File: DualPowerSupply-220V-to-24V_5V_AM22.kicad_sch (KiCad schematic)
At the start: 7 parts, among them U1 AM22-24W2405V

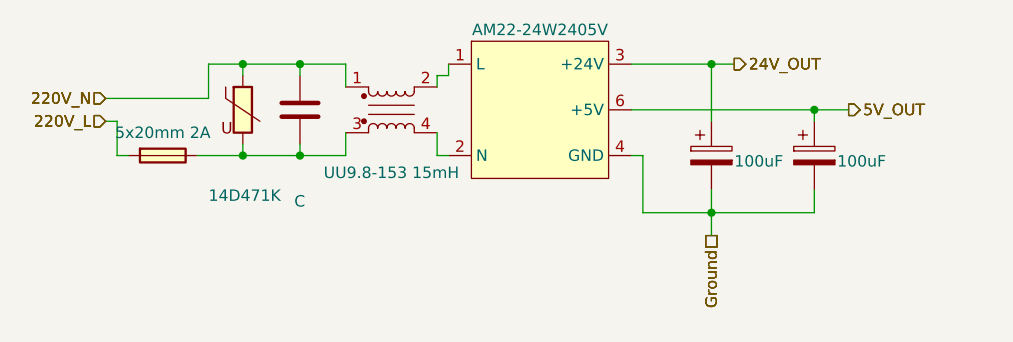
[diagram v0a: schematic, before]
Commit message: layout p1
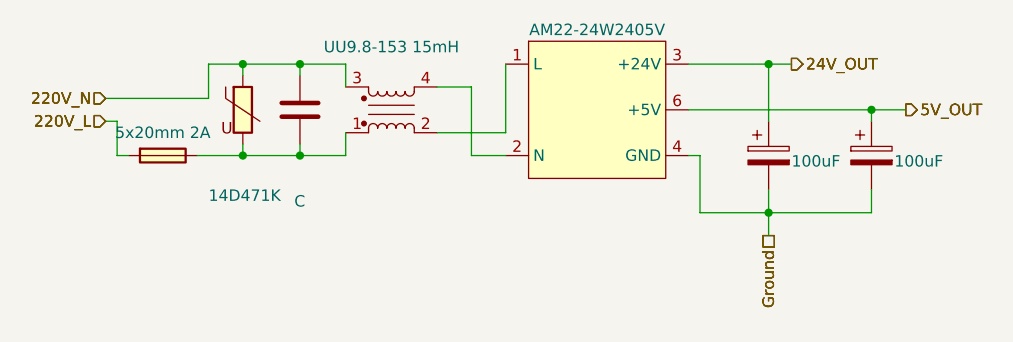
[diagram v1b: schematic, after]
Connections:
- net 220V_N: now also FL1.3; no longer FL1.1
- net at C1.2, F1.2, RV1.2: now also FL1.1; no longer FL1.3
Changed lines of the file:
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@@
 	)
 	(junction
-		(at 157.48 107.95)
+		(at 163.83 107.95)
 		(diameter 0)
 		(color 0 0 0 0)
@@
 	)
 	(junction
-		(at 157.48 91.44)
+		(at 163.83 91.44)
 		(diameter 0)
 		(color 0 0 0 0)
 	)
 	(junction
-		(at 168.91 96.52)
+		(at 175.26 96.52)
 		(diameter 0)
 		(color 0 0 0 0)
@@
 	(wire
 		(pts
-			(xy 127 92.71) (xy 127 93.98)
-		)
-		(stroke
-			(width 0)
-			(type default)
-		)
-	)
-	(wire
-		(pts
-			(xy 148.59 96.52) (xy 168.91 96.52)
+			(xy 154.94 96.52) (xy 175.26 96.52)
 		)
 		(stroke
@@
 	(wire
 		(pts
-			(xy 149.86 107.95) (xy 149.86 101.6)
+			(xy 156.21 107.95) (xy 156.21 101.6)
 		)
 		(stroke
@@
 	(wire
 		(pts
-			(xy 127 92.71) (xy 128.27 92.71)
-		)
-		(stroke
-			(width 0)
-			(type default)
-		)
-	)
-	(wire
-		(pts
-			(xy 160.02 91.44) (xy 157.48 91.44)
-		)
-		(stroke
-			(width 0)
-			(type default)
-		)
-	)
-	(wire
-		(pts
-			(xy 127 99.06) (xy 127 101.6)
-		)
-		(stroke
-			(width 0)
-			(type default)
-		)
-	)
-	(wire
-		(pts
-			(xy 127 101.6) (xy 128.27 101.6)
-		)
-		(stroke
-			(width 0)
-			(type default)
-		)
-	)
-	(wire
-		(pts
-			(xy 128.27 92.71) (xy 128.27 91.44)
+			(xy 166.37 91.44) (xy 163.83 91.44)
+		)
+		(stroke
+			(width 0)
+			(type default)
+		)
+	)
+	(wire
+		(pts
+			(xy 130.81 93.98) (xy 130.81 101.6)
+		)
+		(stroke
+			(width 0)
+			(type default)
+		)
+	)
+	(wire
+		(pts
+			(xy 127 99.06) (xy 134.62 99.06)
 		)
 		(stroke
@@
 	(wire
 		(pts
+			(xy 127 93.98) (xy 130.81 93.98)
+		)
+		(stroke
+			(width 0)
+			(type default)
+		)
+	)
+	(wire
+		(pts
 			(xy 111.76 100.33) (xy 111.76 101.6)
 		)
@@
 	(wire
 		(pts
-			(xy 157.48 91.44) (xy 157.48 97.79)
-		)
-		(stroke
-			(width 0)
-			(type default)
-		)
-	)
-	(wire
-		(pts
-			(xy 168.91 96.52) (xy 168.91 97.79)
+			(xy 163.83 91.44) (xy 163.83 97.79)
+		)
+		(stroke
+			(width 0)
+			(type default)
+		)
+	)
+	(wire
+		(pts
+			(xy 175.26 96.52) (xy 175.26 97.79)
 		)
 		(stroke
@@
 	(wire
 		(pts
-			(xy 157.48 105.41) (xy 157.48 107.95)
-		)
-		(stroke
-			(width 0)
-			(type default)
-		)
-	)
-	(wire
-		(pts
-			(xy 168.91 105.41) (xy 168.91 107.95)
-		)
-		(stroke
-			(width 0)
-			(type default)
-		)
-	)
-	(wire
-		(pts
-			(xy 148.59 91.44) (xy 157.48 91.44)
+			(xy 163.83 105.41) (xy 163.83 107.95)
+		)
+		(stroke
+			(width 0)
+			(type default)
+		)
+	)
+	(wire
+		(pts
+			(xy 175.26 105.41) (xy 175.26 107.95)
+		)
+		(stroke
+			(width 0)
+			(type default)
+		)
+	)
+	(wire
+		(pts
+			(xy 154.94 91.44) (xy 163.83 91.44)
 		)
 		(stroke
@@
 	(wire
 		(pts
-			(xy 157.48 107.95) (xy 157.48 110.49)
+			(xy 163.83 107.95) (xy 163.83 110.49)
+		)
+		(stroke
+			(width 0)
+			(type default)
+		)
+	)
+	(wire
+		(pts
+			(xy 134.62 99.06) (xy 134.62 91.44)
 		)
 		(stroke
@@
 	(wire
 		(pts
-			(xy 168.91 96.52) (xy 172.72 96.52)
-		)
-		(stroke
-			(width 0)
-			(type default)
-		)
-	)
-	(wire
-		(pts
-			(xy 149.86 101.6) (xy 148.59 101.6)
-		)
-		(stroke
-			(width 0)
-			(type default)
-		)
-	)
-	(wire
-		(pts
-			(xy 168.91 107.95) (xy 157.48 107.95)
+			(xy 130.81 101.6) (xy 134.62 101.6)
+		)
+		(stroke
+			(width 0)
+			(type default)
+		)
+	)
+	(wire
+		(pts
+			(xy 175.26 96.52) (xy 179.07 96.52)
+		)
+		(stroke
+			(width 0)
+			(type default)
+		)
+	)
+	(wire
+		(pts
+			(xy 156.21 101.6) (xy 154.94 101.6)
+		)
+		(stroke
+			(width 0)
+			(type default)
+		)
+	)
+	(wire
+		(pts
+			(xy 175.26 107.95) (xy 163.83 107.95)
 		)
 		(stroke
@@
 	(wire
 		(pts
-			(xy 149.86 107.95) (xy 157.48 107.95)
+			(xy 156.21 107.95) (xy 163.83 107.95)
 		)
 		(stroke
@@
 	(hierarchical_label "24V_OUT"
 		(shape output)
-		(at 160.02 91.44 0)
+		(at 166.37 91.44 0)
 		(fields_autoplaced yes)
 		(effects
@@
 	(hierarchical_label "24V_OUT"
 		(shape output)
-		(at 160.02 91.44 0)
+		(at 166.37 91.44 0)
 		(fields_autoplaced yes)
 		(effects
@@
 	(hierarchical_label "Ground"
 		(shape passive)
-		(at 157.48 110.49 270)
+		(at 163.83 110.49 270)
 		(fields_autoplaced yes)
 		(effects
@@
 	(hierarchical_label "Ground"
 		(shape passive)
-		(at 157.48 110.49 270)
+		(at 163.83 110.49 270)
 		(fields_autoplaced yes)
 		(effects
@@
 	(hierarchical_label "5V_OUT"
 		(shape output)
-		(at 172.72 96.52 0)
+		(at 179.07 96.52 0)
 		(fields_autoplaced yes)
 		(effects
@@
 	(hierarchical_label "5V_OUT"
 		(shape output)
-		(at 172.72 96.52 0)
+		(at 179.07 96.52 0)
 		(fields_autoplaced yes)
 		(effects
@@
 		(lib_id "IVS_SYMBOLS:Filter_EMI_LL")
 		(at 121.92 96.52 0)
+		(mirror x)
 		(unit 1)
 		(exclude_from_sim no)
@@
 		(dnp no)
 		(property "Reference" "FL1"
-			(at 121.92 100.965 0)
+			(at 121.92 92.075 0)
 			(effects
 				(font
@@
 		)
 		(property "Value" "UU9.8-153 15mH"
-			(at 121.92 103.505 0)
+			(at 121.92 89.535 0)
 			(effects
 				(font
@@
 		)
 		(property "Footprint" "SpiritBoi_Footprint_Library:ACFilterChoke-UU9.8"
-			(at 121.92 104.14 0)
+			(at 121.92 88.9 0)
 			(effects
 				(font
@@
 		)
 		(property "Datasheet" "~"
-			(at 121.92 95.504 0)
+			(at 121.92 97.536 0)
 			(effects
 				(font
@@
 	(symbol
 		(lib_id "Device:C_Polarized")
-		(at 168.91 101.6 0)
+		(at 175.26 101.6 0)
 		(unit 1)
 		(exclude_from_sim no)
@@
 		(dnp no)
 		(property "Reference" "C3"
-			(at 172.085 100.076 0)
+			(at 178.435 100.076 0)
 			(effects
 				(font
@@
 		)
 		(property "Value" "100uF"
-			(at 171.45 102.235 0)
+			(at 177.8 102.235 0)
 			(effects
 				(font
@@
 		)
 		(property "Footprint" "SpiritBoi_Footprint_Library:CP-Alu-SMD-8x10.5mm"
-			(at 169.8752 105.41 0)
+			(at 176.2252 105.41 0)
 			(effects
 				(font
@@
 		)
 		(property "Datasheet" "~"
-			(at 168.91 101.6 0)
+			(at 175.26 101.6 0)
 			(effects
 				(font
@@
 		)
 		(property "Description" ""
-			(at 168.91 101.6 0)
+			(at 175.26 101.6 0)
 			(effects
 				(font
@@
 	(symbol
 		(lib_id "SpiritBoi_Library:AM22-24W2405V")
-		(at 138.43 96.52 0)
+		(at 144.78 96.52 0)
 		(unit 1)
 		(exclude_from_sim no)
@@
 		(fields_autoplaced yes)
 		(property "Reference" "U1"
-			(at 138.43 85.09 0)
+			(at 144.78 85.09 0)
 			(effects
 				(font
@@
 		)
 		(property "Value" "AM22-24W2405V"
-			(at 138.43 87.63 0)
+			(at 144.78 87.63 0)
 			(effects
 				(font
@@
 		)
 		(property "Footprint" "SpiritBoi_Footprint_Library:DualPowerSupply-24W_24V_05V_AM22"
-			(at 138.43 96.52 0)
+			(at 144.78 96.52 0)
 			(effects
 				(font
@@
 		)
 		(property "Datasheet" ""
-			(at 138.43 96.52 0)
+			(at 144.78 96.52 0)
 			(effects
 				(font
@@
 		)
 		(property "Description" ""
-			(at 138.43 96.52 0)
+			(at 144.78 96.52 0)
 			(effects
 				(font
@@
 	(symbol
 		(lib_id "Device:C_Polarized")
-		(at 157.48 101.6 0)
+		(at 163.83 101.6 0)
 		(unit 1)
 		(exclude_from_sim no)
@@
 		(dnp no)
 		(property "Reference" "C2"
-			(at 160.655 100.076 0)
+			(at 167.005 100.076 0)
 			(effects
 				(font
@@
 		)
 		(property "Value" "100uF"
-			(at 160.02 102.235 0)
+			(at 166.37 102.235 0)
 			(effects
 				(font
@@
 		)
 		(property "Footprint" "SpiritBoi_Footprint_Library:CP-Alu-SMD-8x10.5mm"
-			(at 158.4452 105.41 0)
+			(at 164.7952 105.41 0)
 			(effects
 				(font
@@
 		)
 		(property "Datasheet" "~"
-			(at 157.48 101.6 0)
+			(at 163.83 101.6 0)
 			(effects
 				(font
@@
 		)
 		(property "Description" ""
-			(at 157.48 101.6 0)
-			(effects
-				(font
+			(at 163.83 101.6 0)
+			(effects
+				(font
